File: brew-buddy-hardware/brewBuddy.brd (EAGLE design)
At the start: 44.5 x 75.6 mm, 3 parts

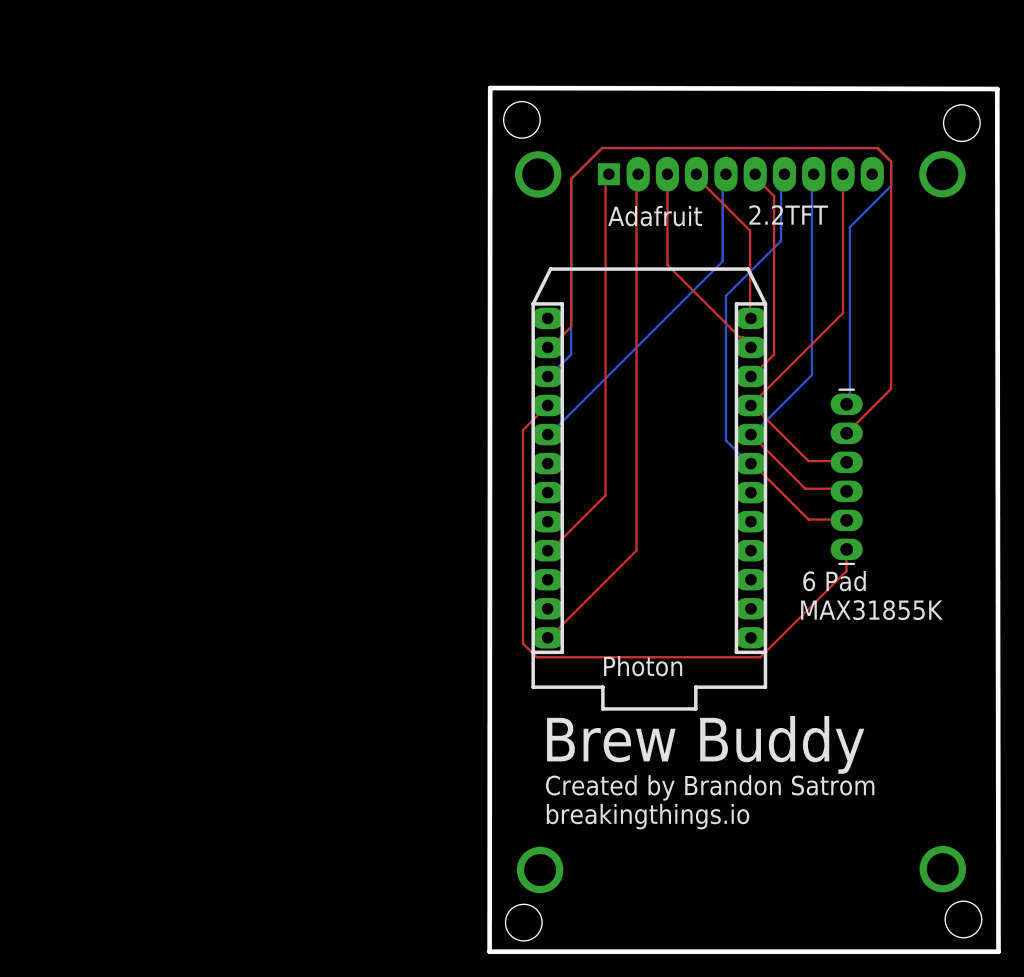
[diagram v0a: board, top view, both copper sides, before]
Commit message: updated schematic and board for Argon
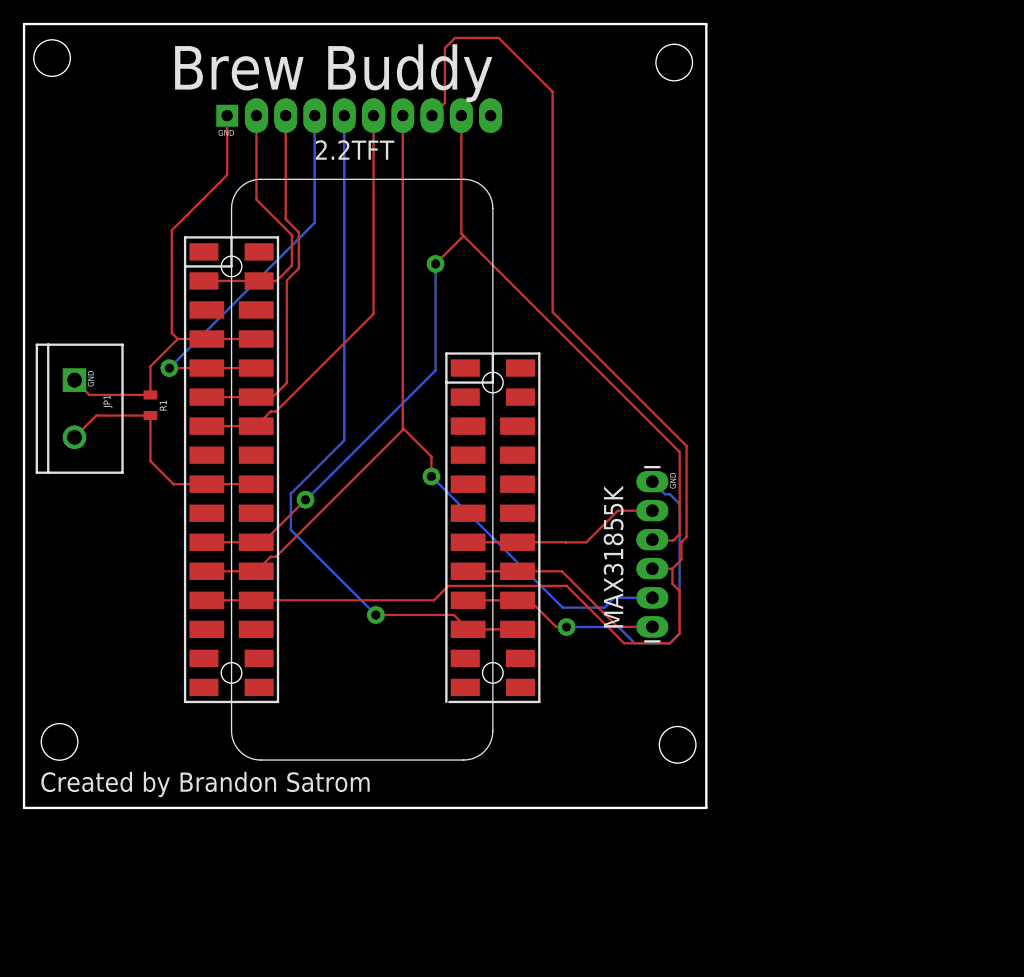
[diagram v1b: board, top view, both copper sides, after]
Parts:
- removed U$1: PHOTON_WITH_HEADERS, Spark:PHOTON
- added JP1: KNOCK, SparkFun-Connectors:SCREWTERMINAL-5MM-2
- added MS1: FEATHERWING_SMTDUAL, Particle-Mesh:FEATHERWING_SMT2
- added R1: 1M, SparkFun-Resistors:0805
- 2.2TFT: value (none) -> TFT
- moved 2.2TFT 33.8 mm to (-12.9, 73.3)
- moved MAX31855K 18.3 mm to (14.3, 41.2)
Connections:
- removed net N$1: MAX31855K.1, U$1.15
- removed net N$10: 2.2TFT.4, U$1.12
- removed net N$11: 2.2TFT.3, U$1.11
- removed net N$12: 2.2TFT.2, U$1.24
- removed net N$13: 2.2TFT.1, U$1.21
- removed net N$2: MAX31855K.2, U$1.14
- removed net N$3: MAX31855K.6, U$1.16
- removed net N$4: 2.2TFT.9, MAX31855K.3, U$1.9
- removed net N$5: 2.2TFT.8, MAX31855K.4, U$1.8
- removed net N$6: 2.2TFT.7, MAX31855K.5, U$1.7
- removed net N$7: 2.2TFT.5, U$1.17
- removed net N$9: 2.2TFT.6, U$1.10
- removed net VBAT: U$1.22
- removed net VIN: U$1.1
- new net 3V3: 2.2TFT.2, MS1.2, MS1.2'
- new net KNOCK: JP1.2, MS1.9, MS1.9', R1.2
- new net MISO: 2.2TFT.8, MAX31855K.4, MS1.13, MS1.13'
- new net MOSI: 2.2TFT.7, MAX31855K.5, MS1.12, MS1.12'
- new net SCK: 2.2TFT.9, MAX31855K.3, MS1.11, MS1.11'
- new net SD_CS: 2.2TFT.5, MS1.19, MS1.19'
- new net TC_CS: MAX31855K.6, MS1.21, MS1.21'
- new net TC_GND: MAX31855K.1, MS1.20, MS1.20'
- new net TFT_CS: 2.2TFT.6, MS1.7, MS1.7'
- new net TFT_DC: 2.2TFT.3, MS1.6, MS1.6'
- new net TFT_RST: 2.2TFT.4, MS1.5, MS1.5'
- new net VCC: MAX31855K.2, MS1.22, MS1.22'
- net GND: now also 2.2TFT.1, JP1.1, MS1.4, MS1.4', R1.1; no longer U$1.2
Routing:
- net MISO: track 0.00 -> 117.2 mm
- net SCK: track 0.00 -> 86.2 mm, vias 0 -> 2
- net MOSI: track 0.00 -> 79.5 mm, vias 0 -> 1
- net N$2: track 70.7 -> 0.00 mm
- net N$1: track 70.7 -> 0.00 mm
- net SD_CS: track 0.00 -> 61.6 mm, vias 0 -> 1
- net N$3: track 55.5 -> 0.00 mm
- net N$12: track 43.9 -> 0.00 mm
- net GND: track 0.00 -> 41.7 mm
- net N$6: track 39.0 -> 0.00 mm
- net TFT_CS: track 0.00 -> 36.0 mm
- net N$5: track 35.7 -> 0.00 mm
- net N$13: track 35.4 -> 0.00 mm
- net TC_GND: track 0.00 -> 35.0 mm, vias 0 -> 1
- net TFT_RST: track 0.00 -> 35.0 mm, vias 0 -> 1
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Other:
- board size 44.5 x 75.6 mm -> 59.7 x 68.6 mm
- board text added: "Created by Brandon Satrom"
- board text added: "GND"
- board text removed: "Adafruit"
- board text removed: "Created by Brandon Satrom breakingthings.io"
- board text removed: "Photon"
- board text removed: "breakingthings.io"
